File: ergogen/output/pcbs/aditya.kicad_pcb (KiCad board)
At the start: 2 copper layers, 133.2 x 110.8 mm, 85 parts

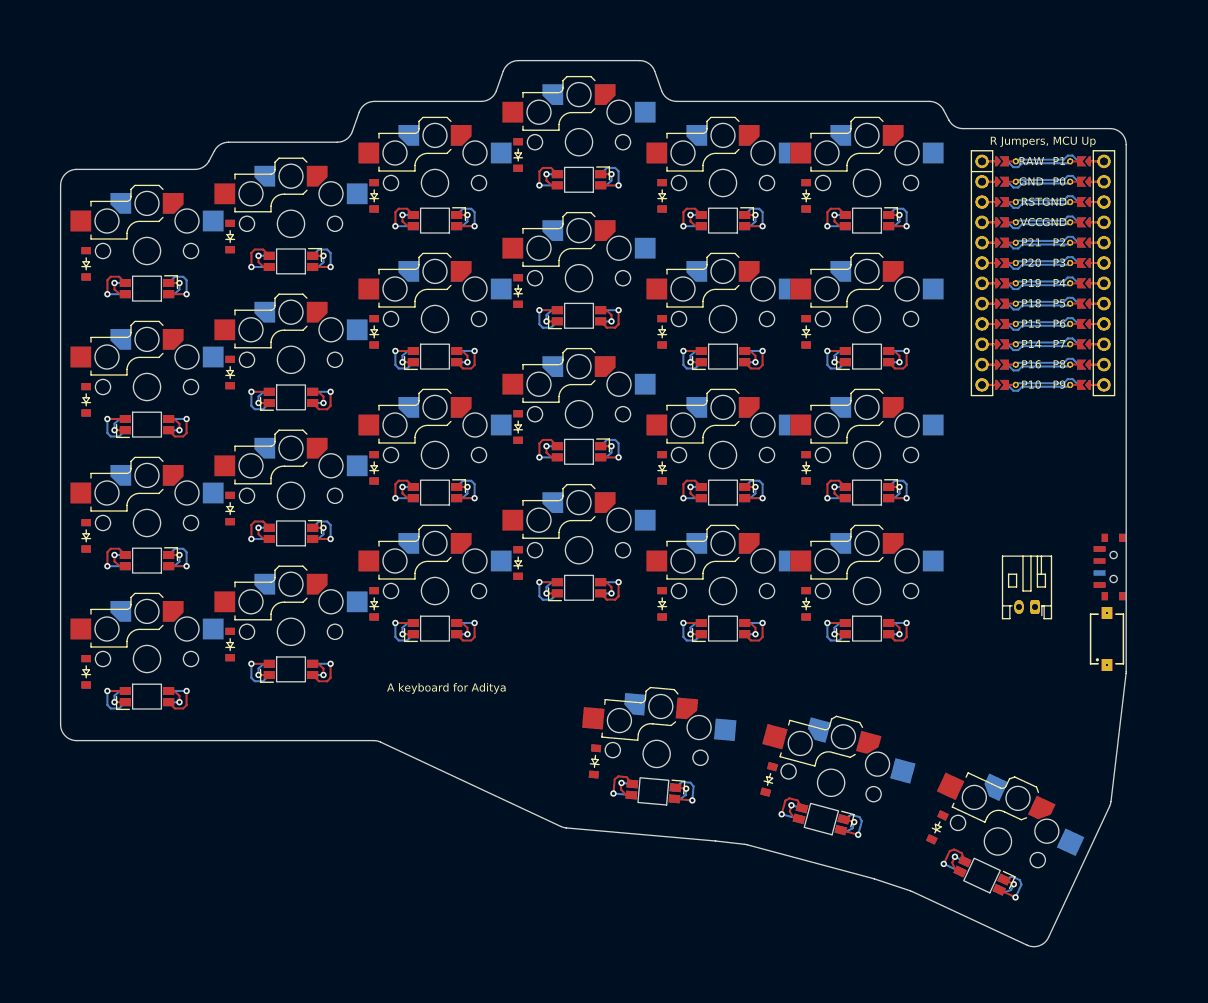
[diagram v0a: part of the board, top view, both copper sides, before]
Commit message: ft. StackOverChonk
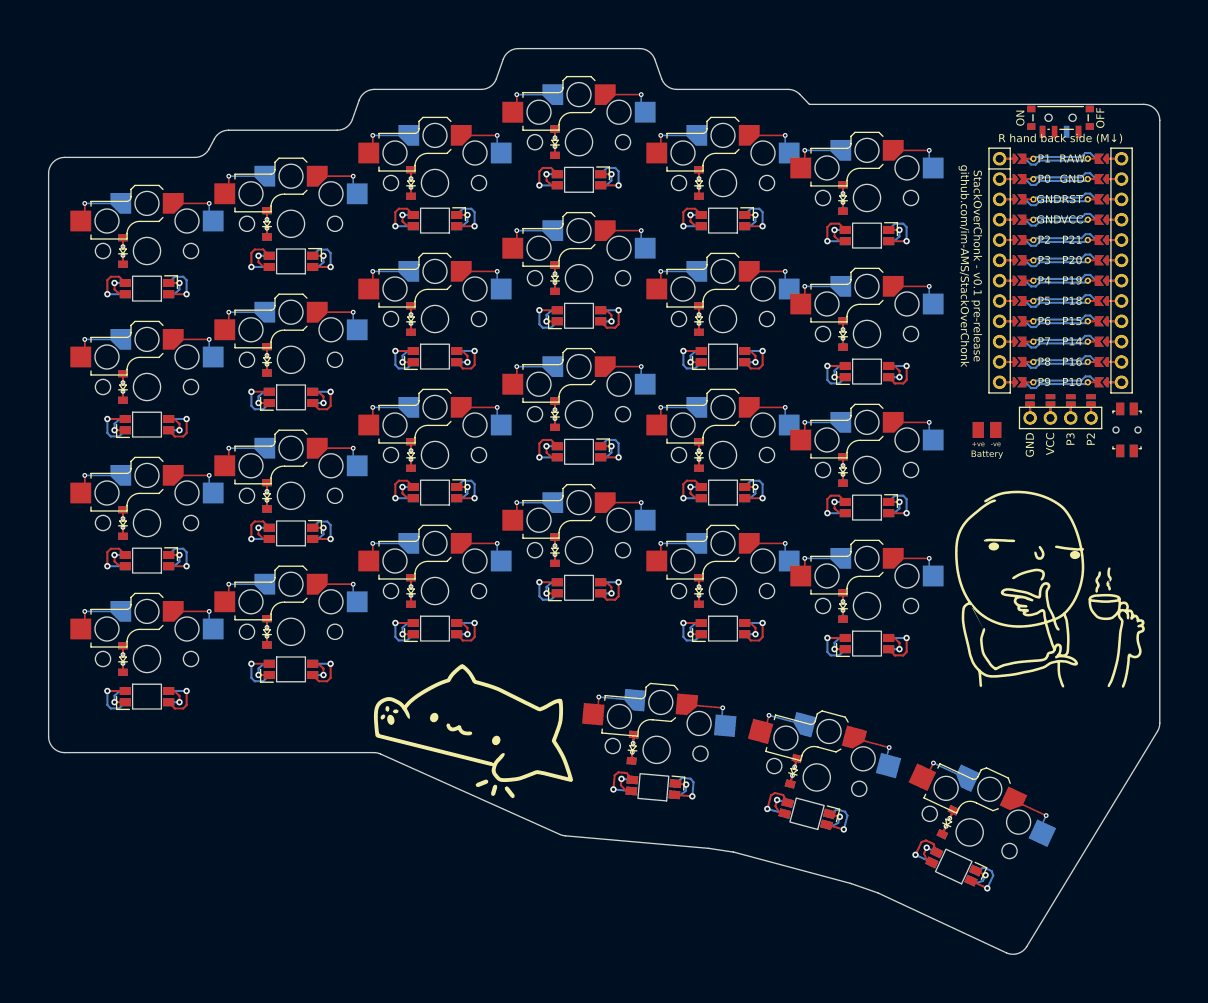
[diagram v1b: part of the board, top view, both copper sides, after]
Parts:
- removed S28: , 434121025816
- removed T1: , Button_Switch_SMD:SW_SPDT_PCM12
- removed _2: , Connector_JST:JST_PH_S2B-PH-K_1x02_P2.00mm_Horizontal
- added BT1: , Battery_pads, F.Cu at (205.0, 71.4)
- added BT2: , Battery_pads, B.Cu at (205.0, 71.4)
- added DISP1: , ceoloide:display_ssd1306, F.Cu at (214.2, 53.2)
- added PWR1: , ceoloide:power_switch_smd_side, B.Cu at (214.2, 32.4)
- added RST1: , ceoloide:reset_switch_smd_side, F.Cu at (222.5, 71.4)
- D1, D10, D11, D12, D13, D14, D15, D16, D17, D18, D19, D2, D20, D21, D22, D23, D24, D25, D26, D27, D3, D4, D5, D6, D7, D8, D9: moved to F.Cu
- moved D25 5.02 mm to (160.7, 111.1)
- moved D11 4.87 mm to (133.0, 57.5)
- moved D12 4.87 mm to (133.0, 40.5)
- moved D15 4.87 mm to (151.0, 52.4)
- moved D16 4.87 mm to (151.0, 35.4)
- moved D19 4.87 mm to (169.0, 57.5)
- moved D20 4.87 mm to (169.0, 40.5)
- moved D4 4.87 mm to (97.0, 49.0)
- moved D8 4.87 mm to (115.0, 45.6)
- moved D1 4.87 mm to (97.0, 100.0)
- moved D10 4.87 mm to (133.0, 74.5)
- moved D13 4.87 mm to (151.0, 86.4)
- moved D14 4.87 mm to (151.0, 69.4)
- moved D17 4.87 mm to (169.0, 91.5)
- moved D18 4.87 mm to (169.0, 74.5)
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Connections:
- D25 pad 1: P10 -> P7
- D26 pad 1: P10 -> P7
- D27 pad 1: P10 -> P7
- MCU1 pad 101: P1 -> RAW
- MCU1 pad 102: P0 -> GND
- MCU1 pad 103: GND -> RST
- MCU1 pad 104: GND -> VCC
- MCU1 pad 105: P2 -> P21
- MCU1 pad 106: P3 -> P20
- MCU1 pad 107: P4 -> P19
- MCU1 pad 108: P5 -> P18
- MCU1 pad 109: P6 -> P15
- MCU1 pad 110: P7 -> P14
- MCU1 pad 111: P8 -> P16
- MCU1 pad 112: P9 -> P10
- MCU1 pad 113: P10 -> P9
- MCU1 pad 114: P16 -> P8
- MCU1 pad 115: P14 -> P7
- MCU1 pad 116: P15 -> P6
- MCU1 pad 117: P18 -> P5
- MCU1 pad 118: P19 -> P4
- MCU1 pad 119: P20 -> P3
- MCU1 pad 120: P21 -> P2
- MCU1 pad 121: VCC -> GND
- MCU1 pad 122: RST -> GND
- MCU1 pad 123: GND -> P0
- MCU1 pad 124: RAW -> P1
- S1 pad 1: P1 -> matrix_outer_down
- S1 pad 2: matrix_outer_down -> P1
- S10 pad 1: P4 -> matrix_ring_home
- S10 pad 2: matrix_ring_home -> P4
- S11 pad 1: P4 -> matrix_ring_up
- S11 pad 2: matrix_ring_up -> P4
- S12 pad 1: P4 -> matrix_ring_num
- S12 pad 2: matrix_ring_num -> P4
- S13 pad 1: P5 -> matrix_middle_down
- S13 pad 2: matrix_middle_down -> P5
- S14 pad 1: P5 -> matrix_middle_home
- S14 pad 2: matrix_middle_home -> P5
- S15 pad 1: P5 -> matrix_middle_up
- S15 pad 2: matrix_middle_up -> P5
- S16 pad 1: P5 -> matrix_middle_num
- S16 pad 2: matrix_middle_num -> P5
- S17 pad 1: P7 -> matrix_index_down
- S17 pad 2: matrix_index_down -> P7
- S18 pad 1: P7 -> matrix_index_home
- S18 pad 2: matrix_index_home -> P7
- S19 pad 1: P7 -> matrix_index_up
- S19 pad 2: matrix_index_up -> P7
- S2 pad 1: P1 -> matrix_outer_home
- S2 pad 2: matrix_outer_home -> P1
- S20 pad 1: P7 -> matrix_index_num
- S20 pad 2: matrix_index_num -> P7
- S21 pad 1: P8 -> matrix_inner_down
- S21 pad 2: matrix_inner_down -> P8
- S22 pad 1: P8 -> matrix_inner_home
- S22 pad 2: matrix_inner_home -> P8
- S23 pad 1: P8 -> matrix_inner_up
- S23 pad 2: matrix_inner_up -> P8
- S24 pad 1: P8 -> matrix_inner_num
- S24 pad 2: matrix_inner_num -> P8
- S25 pad 1: P7 -> thumbs_col1_cluster
- S25 pad 2: thumbs_col1_cluster -> P5
- S26 pad 1: P8 -> thumbs_col2_cluster
- S26 pad 2: thumbs_col2_cluster -> P7
- S27 pad 1: P9 -> thumbs_col3_cluster
- S27 pad 2: thumbs_col3_cluster -> P8
- S3 pad 1: P1 -> matrix_outer_up
- S3 pad 2: matrix_outer_up -> P1
- S4 pad 1: P1 -> matrix_outer_num
- S4 pad 2: matrix_outer_num -> P1
- S5 pad 1: P0 -> matrix_pinky_down
- S5 pad 2: matrix_pinky_down -> P0
- S6 pad 1: P0 -> matrix_pinky_home
- S6 pad 2: matrix_pinky_home -> P0
- S7 pad 1: P0 -> matrix_pinky_up
- S7 pad 2: matrix_pinky_up -> P0
- S8 pad 1: P0 -> matrix_pinky_num
- S8 pad 2: matrix_pinky_num -> P0
- S9 pad 1: P4 -> matrix_ring_down
- S9 pad 2: matrix_ring_down -> P4
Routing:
- net P7: track 0.00 -> 40.1 mm, vias 0 -> 8
- net P5: track 0.00 -> 33.5 mm, vias 0 -> 5
- net P8: track 0.00 -> 33.5 mm, vias 0 -> 5
- net P4: track 0.00 -> 26.8 mm, vias 0 -> 4
- net P1: track 0.00 -> 26.8 mm, vias 0 -> 4
- net P0: track 0.00 -> 26.8 mm, vias 0 -> 4
- net P19: track 0.00 -> 13.2 mm, vias 0 -> 6
- net P18: track 0.00 -> 13.2 mm, vias 0 -> 6
- net P20: track 0.00 -> 13.2 mm, vias 0 -> 6
- net P21: track 0.00 -> 13.2 mm, vias 0 -> 6
- net thumbs_col1_cluster: track 0.00 -> 8.90 mm, vias 0 -> 2
- net matrix_ring_home: track 0.00 -> 8.90 mm, vias 0 -> 2
- net matrix_ring_down: track 0.00 -> 8.90 mm, vias 0 -> 2
- net matrix_pinky_home: track 0.00 -> 8.90 mm, vias 0 -> 2
- net matrix_pinky_down: track 0.00 -> 8.90 mm, vias 0 -> 2
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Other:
- board size 133.2 x 110.8 mm -> 138.9 x 113.2 mm
- board text added: "StackOverChonk - v0.1 pre-release github.com/im-AMS/StackOverChonk"
- board text removed: "A keyboard for Aditya"
